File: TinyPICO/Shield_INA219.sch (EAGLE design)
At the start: 11 parts, among them J1 3.5mm, U1 INA219BIDCNT

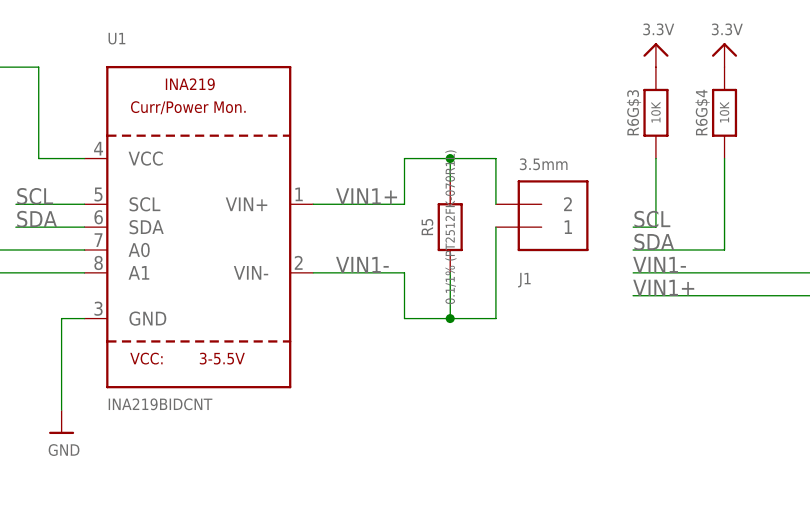
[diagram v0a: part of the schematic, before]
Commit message: Prettied up the boards a little
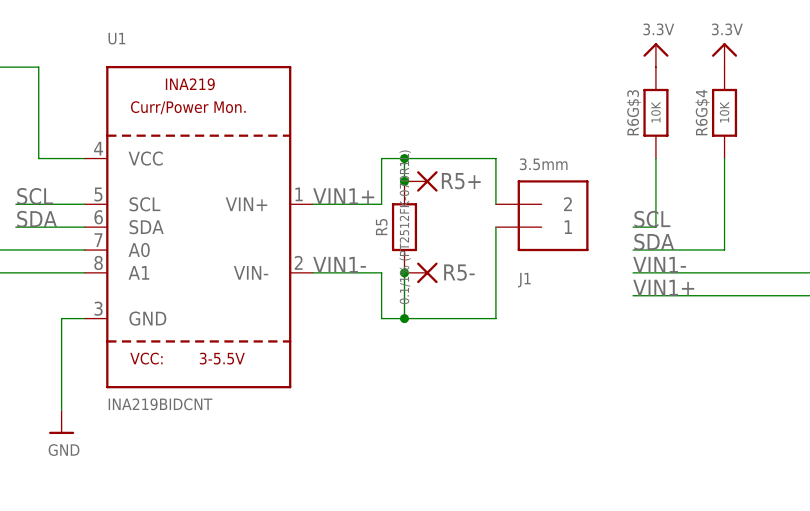
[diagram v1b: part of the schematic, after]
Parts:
- added R5+, R5-: (no value), wirepad:1,6/0,9
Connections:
- net VIN1+: now also R5+.P
- net VIN1-: now also R5-.P
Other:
- moved on the sheet: R5
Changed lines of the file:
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@@
 <part name="JP2" library="microbuilder" deviceset="HEADER-1X2" device="ROUND"/>
 <part name="R6" library="microbuilder" deviceset="RESISTOR_4PACK" device="" value="10K"/>
+<part name="R5+" library="wirepad" library_urn="urn:adsk.eagle:library:412" deviceset="1,6/0,9" device="" package3d_urn="urn:adsk.eagle:package:30840/1"/>
+<part name="R5-" library="wirepad" library_urn="urn:adsk.eagle:library:412" deviceset="1,6/0,9" device="" package3d_urn="urn:adsk.eagle:package:30840/1"/>
 </parts>
 <sheets>
@@
 <attribute name="VALUE" x="51.816" y="134.62" size="1.27" layer="96"/>
 </instance>
-<instance part="R5" gate="G$1" x="119.38" y="134.62" smashed="yes" rot="R90">
-<attribute name="NAME" x="116.84" y="134.62" size="1.27" layer="95" font="vector" rot="R90" align="center"/>
-<attribute name="VALUE" x="119.38" y="134.62" size="1.016" layer="96" font="vector" ratio="15" rot="R90" align="center"/>
+<instance part="R5" gate="G$1" x="114.3" y="134.62" smashed="yes" rot="R90">
+<attribute name="NAME" x="111.76" y="134.62" size="1.27" layer="95" font="vector" rot="R90" align="center"/>
+<attribute name="VALUE" x="114.3" y="134.62" size="1.016" layer="96" font="vector" ratio="15" rot="R90" align="center"/>
 </instance>
 <instance part="J1" gate="G$1" x="129.54" y="137.16" smashed="yes" rot="MR180">
@@
 <attribute name="NAME" x="58.42" y="121.92" size="1.27" layer="95" font="vector" rot="R270" align="center"/>
 <attribute name="VALUE" x="55.88" y="121.92" size="1.016" layer="96" font="vector" ratio="15" rot="R270" align="center"/>
+</instance>
+<instance part="R5+" gate="1" x="116.84" y="139.7" smashed="yes" rot="R180">
+<attribute name="NAME" x="118.237" y="138.8618" size="1.778" layer="95"/>
+<attribute name="VALUE" x="117.983" y="143.002" size="1.778" layer="96" rot="R180"/>
+</instance>
+<instance part="R5-" gate="1" x="116.84" y="129.54" smashed="yes" rot="R180">
+<attribute name="NAME" x="118.491" y="128.7018" size="1.778" layer="95"/>
+<attribute name="VALUE" x="117.983" y="132.842" size="1.778" layer="96" rot="R180"/>
 </instance>
 </instances>
@@
 <net name="VIN1+" class="0">
 <segment>
-<wire x1="104.14" y1="137.16" x2="114.3" y2="137.16" width="0.1524" layer="91"/>
-<wire x1="114.3" y1="137.16" x2="114.3" y2="142.24" width="0.1524" layer="91"/>
-<wire x1="114.3" y1="142.24" x2="119.38" y2="142.24" width="0.1524" layer="91"/>
-<wire x1="119.38" y1="142.24" x2="119.38" y2="139.7" width="0.1524" layer="91"/>
-<label x="106.68" y="137.16" size="1.778" layer="95"/>
+<wire x1="104.14" y1="137.16" x2="111.76" y2="137.16" width="0.1524" layer="91"/>
+<wire x1="111.76" y1="137.16" x2="111.76" y2="142.24" width="0.1524" layer="91"/>
+<wire x1="111.76" y1="142.24" x2="114.3" y2="142.24" width="0.1524" layer="91"/>
+<wire x1="114.3" y1="142.24" x2="114.3" y2="139.7" width="0.1524" layer="91"/>
+<label x="104.14" y="137.16" size="1.778" layer="95"/>
 <pinref part="U1" gate="G$1" pin="VIN+"/>
 <pinref part="R5" gate="G$1" pin="2"/>
-<junction x="119.38" y="142.24"/>
+<junction x="114.3" y="142.24"/>
 <pinref part="J1" gate="G$1" pin="2"/>
-<wire x1="124.46" y1="142.24" x2="119.38" y2="142.24" width="0.1524" layer="91"/>
+<wire x1="124.46" y1="142.24" x2="114.3" y2="142.24" width="0.1524" layer="91"/>
 <wire x1="124.46" y1="137.16" x2="124.46" y2="142.24" width="0.1524" layer="91"/>
+<pinref part="R5+" gate="1" pin="P"/>
+<junction x="114.3" y="139.7"/>
 </segment>
 <segment>
@@
 <net name="VIN1-" class="0">
 <segment>
-<wire x1="104.14" y1="129.54" x2="114.3" y2="129.54" width="0.1524" layer="91"/>
-<wire x1="114.3" y1="129.54" x2="114.3" y2="124.46" width="0.1524" layer="91"/>
-<wire x1="114.3" y1="124.46" x2="119.38" y2="124.46" width="0.1524" layer="91"/>
-<wire x1="119.38" y1="124.46" x2="119.38" y2="129.54" width="0.1524" layer="91"/>
-<label x="106.68" y="129.54" size="1.778" layer="95"/>
+<wire x1="104.14" y1="129.54" x2="111.76" y2="129.54" width="0.1524" layer="91"/>
+<wire x1="111.76" y1="129.54" x2="111.76" y2="124.46" width="0.1524" layer="91"/>
+<wire x1="111.76" y1="124.46" x2="114.3" y2="124.46" width="0.1524" layer="91"/>
+<wire x1="114.3" y1="124.46" x2="114.3" y2="129.54" width="0.1524" layer="91"/>
+<label x="104.14" y="129.54" size="1.778" layer="95"/>
 <pinref part="U1" gate="G$1" pin="VIN-"/>
 <pinref part="R5" gate="G$1" pin="1"/>
-<junction x="119.38" y="124.46"/>
+<junction x="114.3" y="124.46"/>
 <pinref part="J1" gate="G$1" pin="1"/>
-<wire x1="119.38" y1="124.46" x2="124.46" y2="124.46" width="0.1524" layer="91"/>
+<wire x1="114.3" y1="124.46" x2="124.46" y2="124.46" width="0.1524" layer="91"/>
 <wire x1="124.46" y1="124.46" x2="124.46" y2="134.62" width="0.1524" layer="91"/>
-</segment>
-<segment>
+<pinref part="R5-" gate="1" pin="P"/>
+<junction x="114.3" y="129.54"/>
+</segment>
+<segment>
